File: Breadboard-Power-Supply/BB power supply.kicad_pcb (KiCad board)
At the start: 2 copper layers, 31.2 x 55.1 mm, 18 parts, among them J1 Conn_01x02_Pin, J2 Conn_01x02_Pin, J3 Conn_01x03_Pin, J4 Conn_01x03_Pin, J5 Screw_Terminal_01x02, J6 Screw_Terminal_01x02, J7 Barrel_Jack_Switch, U1 LM7805_TO220, U2 LM317_TO-220

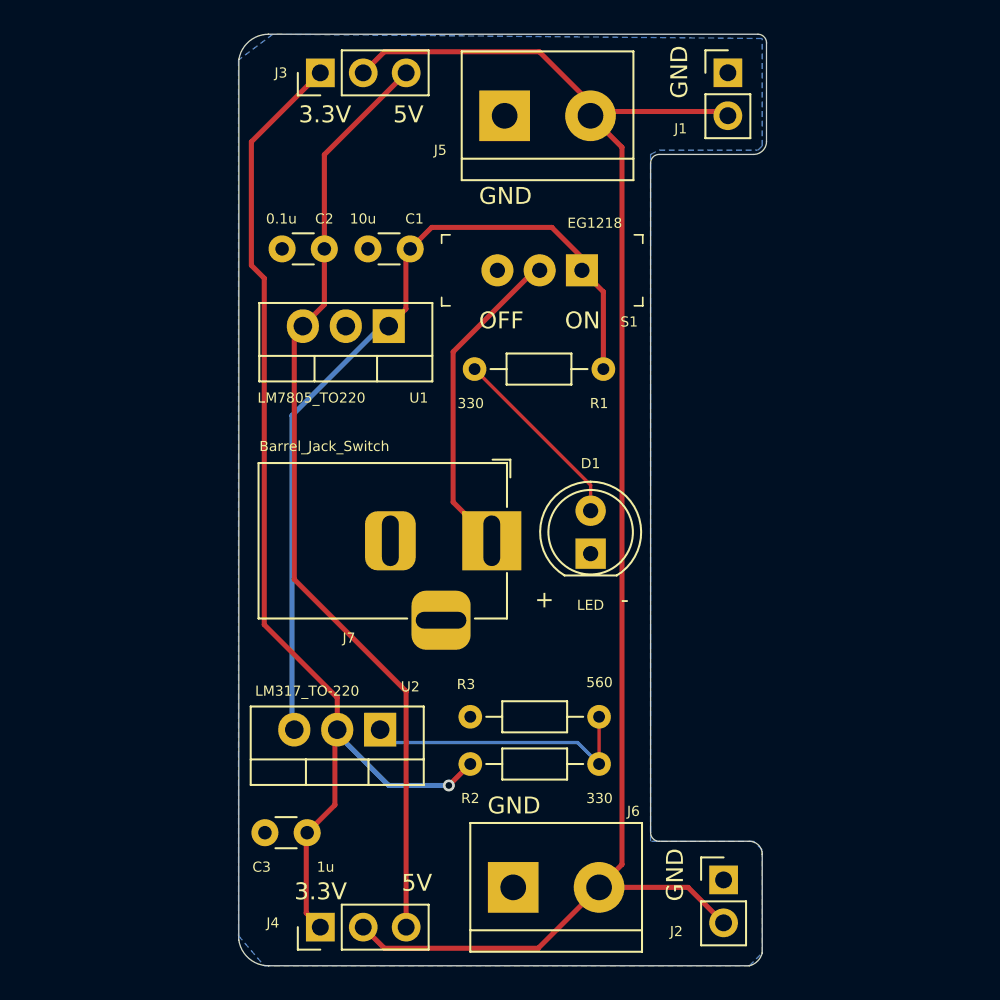
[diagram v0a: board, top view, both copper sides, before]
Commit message: Completed project & Updated
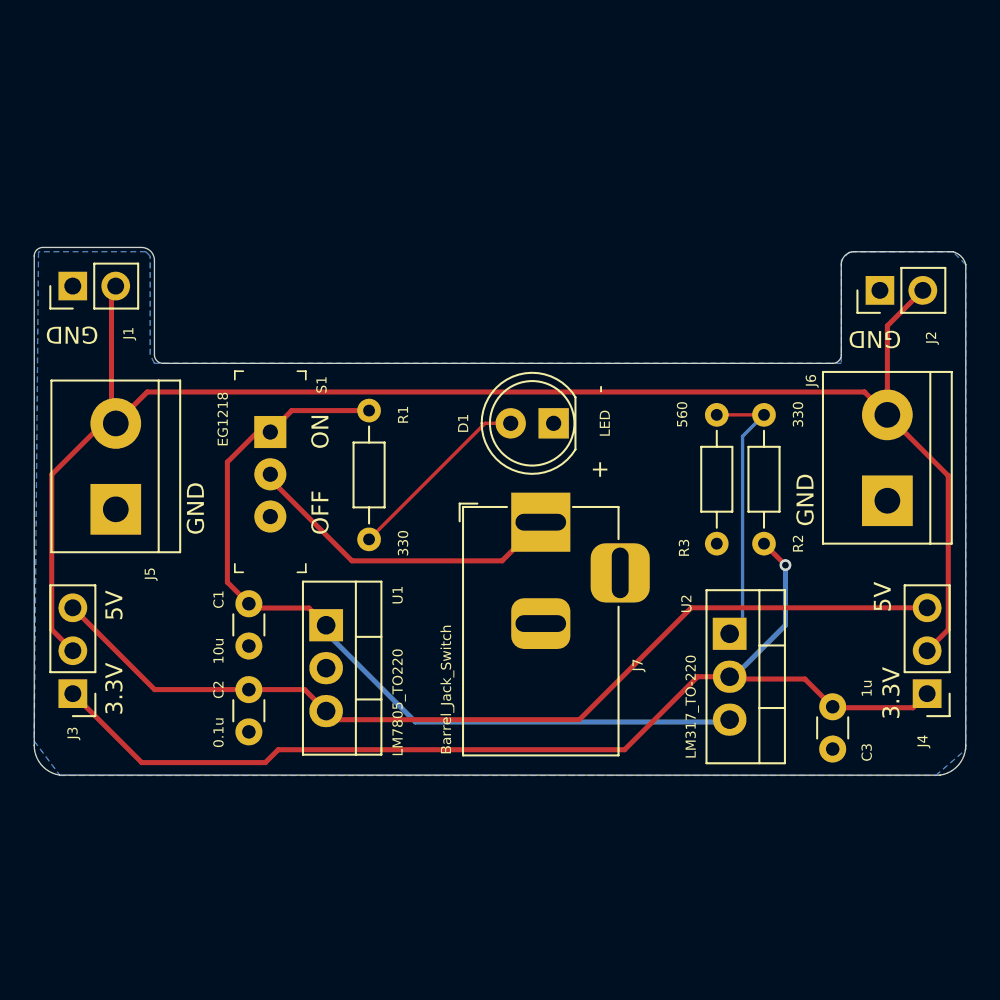
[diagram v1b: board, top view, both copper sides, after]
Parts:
- moved J1 40.8 mm to (129.9, 85.3), turned to 90 degrees
- moved J3 39.5 mm to (129.9, 109.4), turned to 180 degrees
- moved J4 38.5 mm to (180.4, 109.4), turned to 180 degrees
- moved J2 36.1 mm to (177.7, 85.5), turned to 90 degrees
- moved J5 32.7 mm to (132.4, 98.5), turned to 90 degrees
- moved C3 32.0 mm to (174.9, 110.2), turned to -90 degrees
- moved J6 31.8 mm to (178.1, 98.0), turned to 90 degrees
- moved C2 26.5 mm to (140.3, 109.1), turned to -90 degrees
- moved C1 23.1 mm to (140.3, 104.1), turned to -90 degrees
- moved R2 22.8 mm to (170.8, 92.9), turned to -90 degrees
- moved U2 21.4 mm to (168.8, 105.8), turned to -90 degrees
- moved S1 20.8 mm to (141.6, 93.9), turned to -90 degrees
- moved U1 18.1 mm to (144.9, 105.3), turned to -90 degrees
- moved R3 17.8 mm to (168.0, 100.5), turned to 90 degrees
- moved REF** 16.6 mm to (167.2, 96.9), turned to 0 degrees
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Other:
- board size 31.2 x 55.1 mm -> 55.1 x 31.2 mm
